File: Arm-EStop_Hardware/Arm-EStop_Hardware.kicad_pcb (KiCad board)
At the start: 2 copper layers, 86.4 x 48.3 mm, 29 parts, among them Q1 IRFS7437TRLPBFCT, Q2 IRFS7437TRLPBFCT, U1 3.3V, U2 LT1910, U3 LT1910, U4 E_STOP, U5 E_STOP+LED

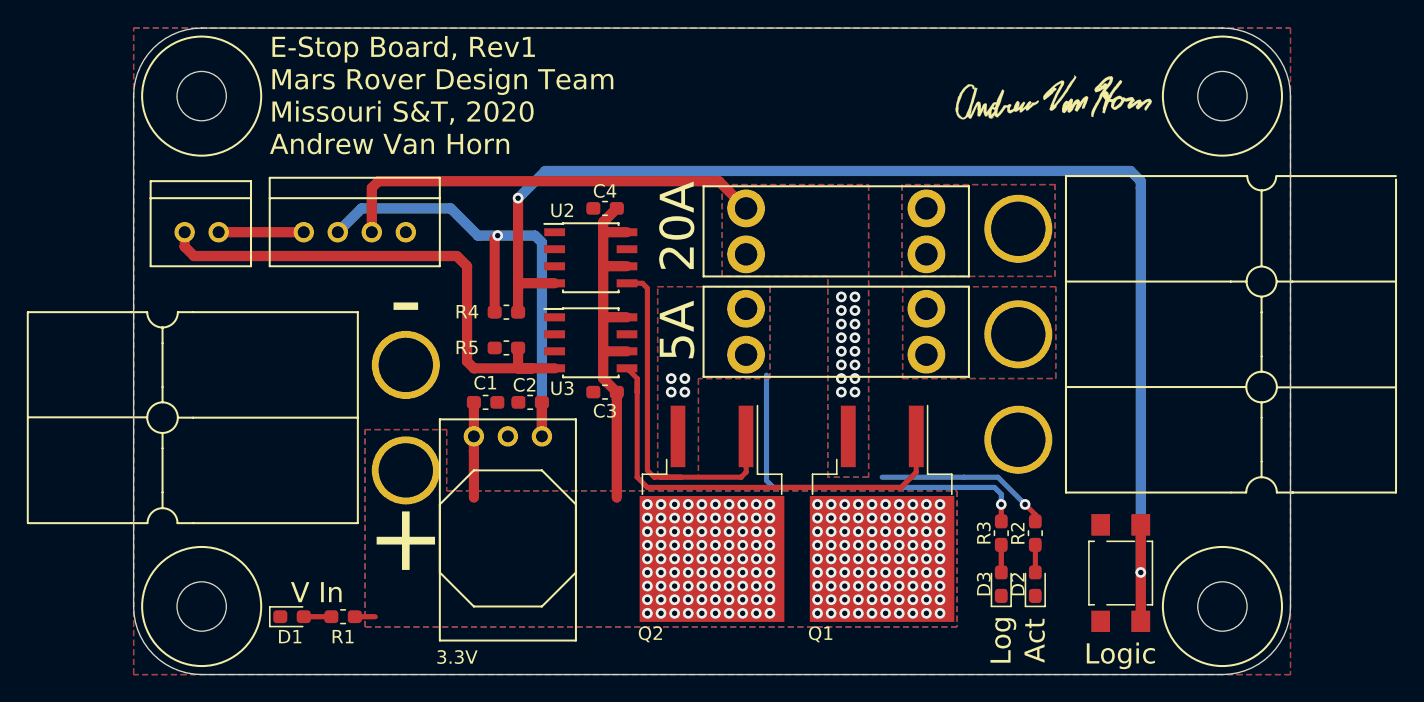
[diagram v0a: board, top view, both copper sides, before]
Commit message: Final changes before PRR
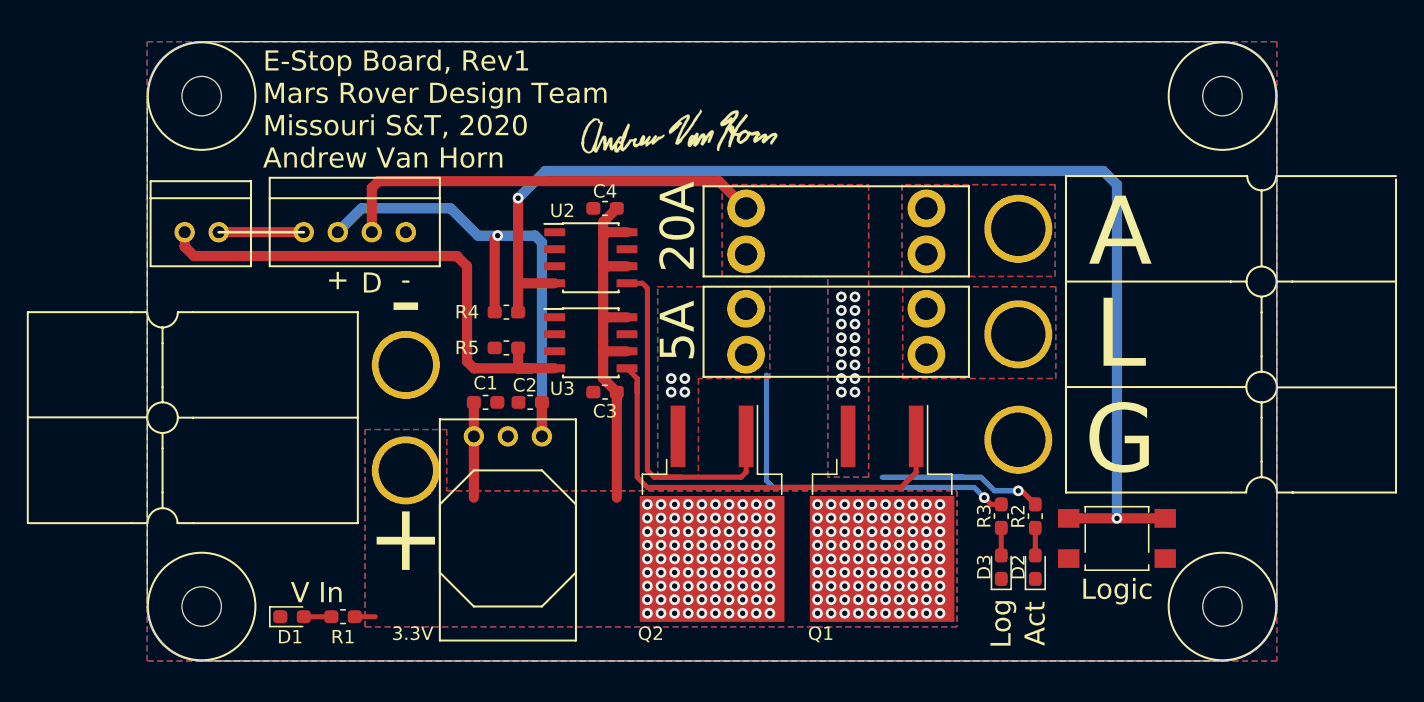
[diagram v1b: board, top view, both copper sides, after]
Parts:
- removed the REF** at (214.0, 95.9)
- removed the REF** at (146.7, 95.9)
- removed the REF** at (146.7, 125.1)
- removed the REF** at (214.0, 125.1)
- added REF**: 4_40_Hole, MRDT_Drill_Holes:4_40_Hole_Corner, F.Cu at (214.4, 125.5)
- added REF**: 4_40_Hole, MRDT_Drill_Holes:4_40_Hole_Corner, F.Cu at (146.2, 125.5)
- added REF**: 4_40_Hole, MRDT_Drill_Holes:4_40_Hole_Corner, F.Cu at (146.2, 95.4)
- added REF**: 4_40_Hole, MRDT_Drill_Holes:4_40_Hole_Corner, F.Cu at (214.4, 95.4)
- moved G*** 28.1 mm to (177.8, 94.0)
- moved Logic 2.60 mm to (210.6, 124.5), turned to 0 degrees
- moved D2 1.27 mm to (204.5, 126.6)
- moved D3 1.27 mm to (201.9, 126.6)
- moved R2 1.27 mm to (204.5, 122.8)
- moved R3 1.27 mm to (201.9, 122.8)
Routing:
- net Net-(R4-Pad2): track 95.3 -> 89.3 mm
- net V_Out_Log: track 27.9 -> 26.1 mm
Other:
- board size 86.4 x 48.3 mm -> 84.3 x 46.2 mm
- board text added: "A"
- board text added: "D"
- board text added: "G"
- board text added: "L"
